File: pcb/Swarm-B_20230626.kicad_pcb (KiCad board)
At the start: 2 copper layers, 81.8 x 72.1 mm, 29 parts, among them J1 5v_3Pi, J2 GND_3Pi, J3 RX_Break, J4 Conn_02x15_Top_Bottom, J5 I2C_3Pi, J6 3PI_SWTCH, J7 I2C_Exp, J8 ProxA, J9 ProxB, U1 74LS32, U2 TSDP34138, U3 TSDP34138, U4 TSDP34138, U5 TSDP34138

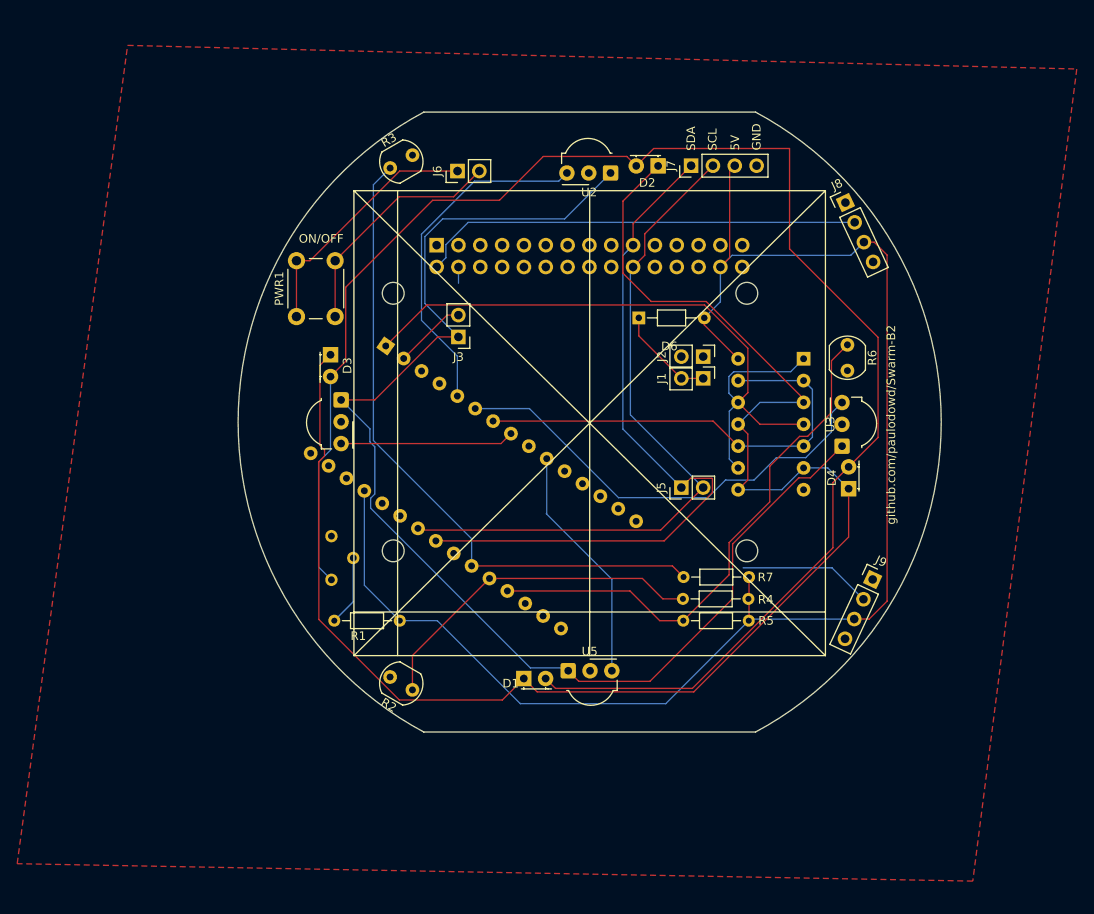
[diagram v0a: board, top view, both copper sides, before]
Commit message: update
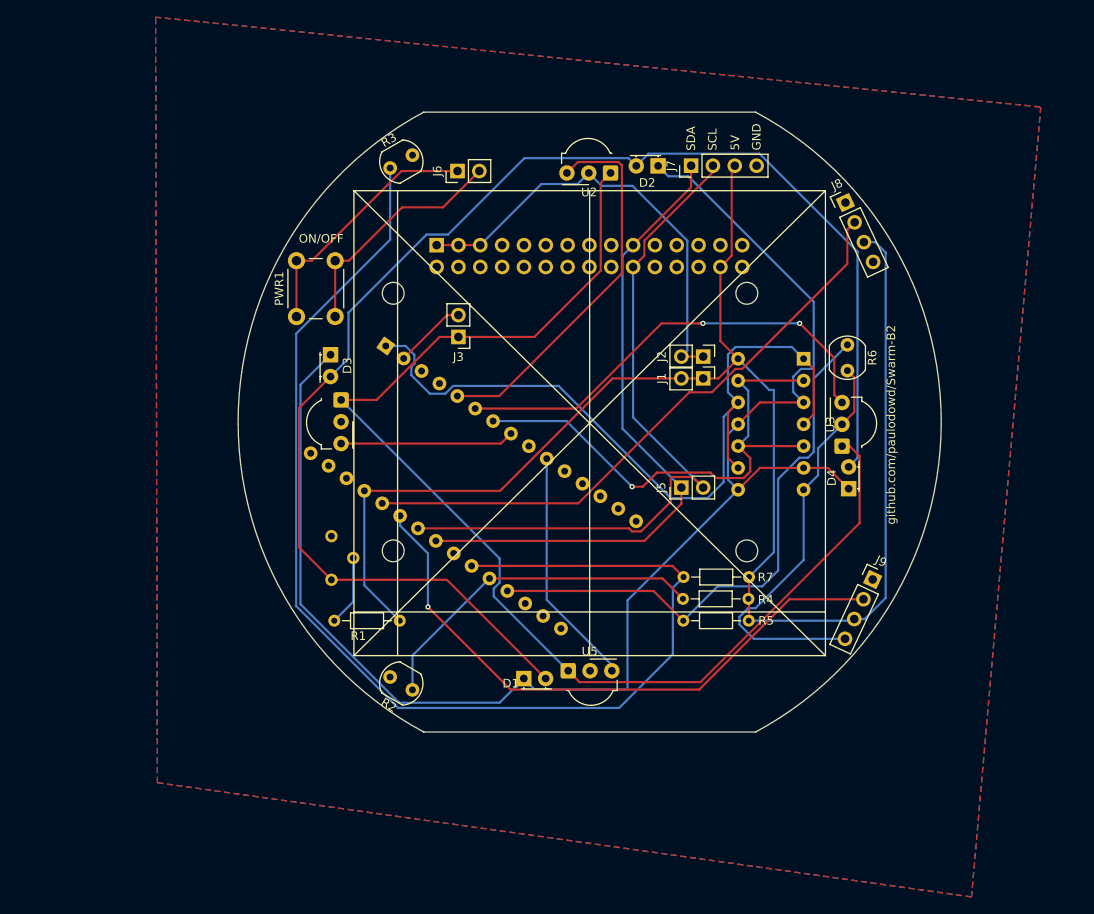
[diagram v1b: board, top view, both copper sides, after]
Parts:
- removed D6: 1N5819, Diode_THT:D_DO-34_SOD68_P7.62mm_Horizontal
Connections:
- A1 pad 25: unconnected-(A1-A6-Pad25) -> Net-(A1-A6)
- A1 pad 26: unconnected-(A1-A7-Pad26) -> Net-(A1-A7)
- J1 pad 1: Net-(D6-K) -> +5V
- J1 pad 2: Net-(D6-K) -> +5V
- J4 pad 2: Net-(J4-Pin_2) -> unconnected-(J4-Pin_2-Pad2)
- J4 pad 4: Net-(J4-Pin_4) -> unconnected-(J4-Pin_4-Pad4)
- J8 pad 2: Net-(J4-Pin_2) -> Net-(A1-A7)
- J9 pad 2: Net-(J4-Pin_4) -> Net-(A1-A6)
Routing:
- net GND: track 0.00 -> 101.1 mm
- net Net-(A1-A6): track 0.00 -> 71.0 mm, vias 0 -> 1
- net Net-(A1-A7): track 0.00 -> 70.9 mm
- net Net-(A1-A2): track 77.0 -> 141.5 mm
- net Net-(J4-Pin_2): track 51.7 -> 0.00 mm
- net Net-(D1-A): track 188.8 -> 162.6 mm
- net Net-(J4-Pin_4): track 17.4 -> 0.00 mm
- net Net-(D1-K): track 186.8 -> 174.5 mm
- net Net-(D6-K): track 11.6 -> 0.00 mm
- net +5V: track 174.6 -> 184.7 mm
- net Net-(A1-D1/TX): track 83.1 -> 93.0 mm
- net Net-(A1-D4): track 53.4 -> 62.1 mm, vias 0 -> 1
- net Net-(A1-A4): track 83.8 -> 75.9 mm
- net Net-(A1-D2): track 40.4 -> 44.7 mm
- net Net-(U2-OUT): track 147.3 -> 143.8 mm
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- added copper zone on B.Cu, net GND
